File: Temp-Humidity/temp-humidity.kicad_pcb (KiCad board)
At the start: 2 copper layers, 34 x 74 mm, 30 parts, among them IC1 ATMEGA328P-A, P1 BATTERY, P2 CONN_02X03, P3 SERIAL/DEBUG, P4 ANTENNA, SW1 SW_PUSH_SMALL_H, U1 AT25DF512, U2 HDC1080, U3 ATSHA204A, U4 NRF24L01, U5 RFM69HW, Y1 12MHz

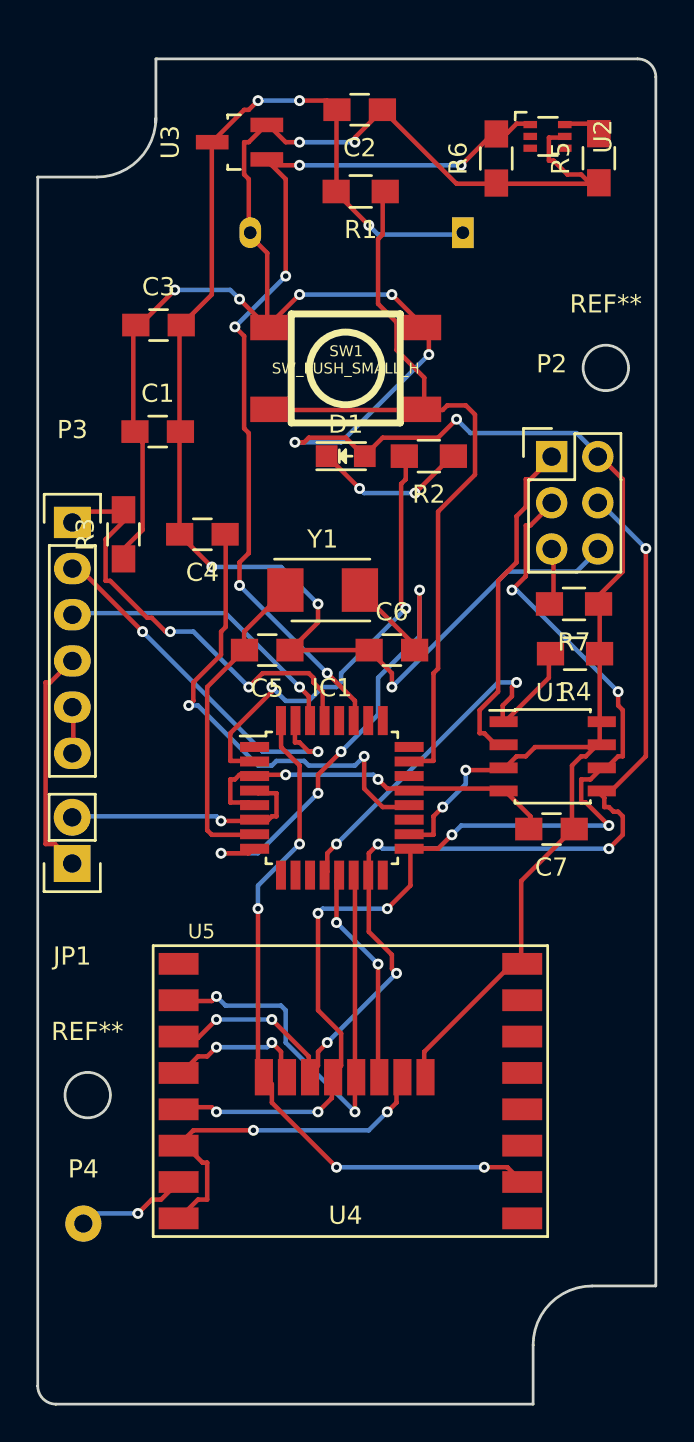
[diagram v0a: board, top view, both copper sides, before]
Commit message: More work on hum/temp
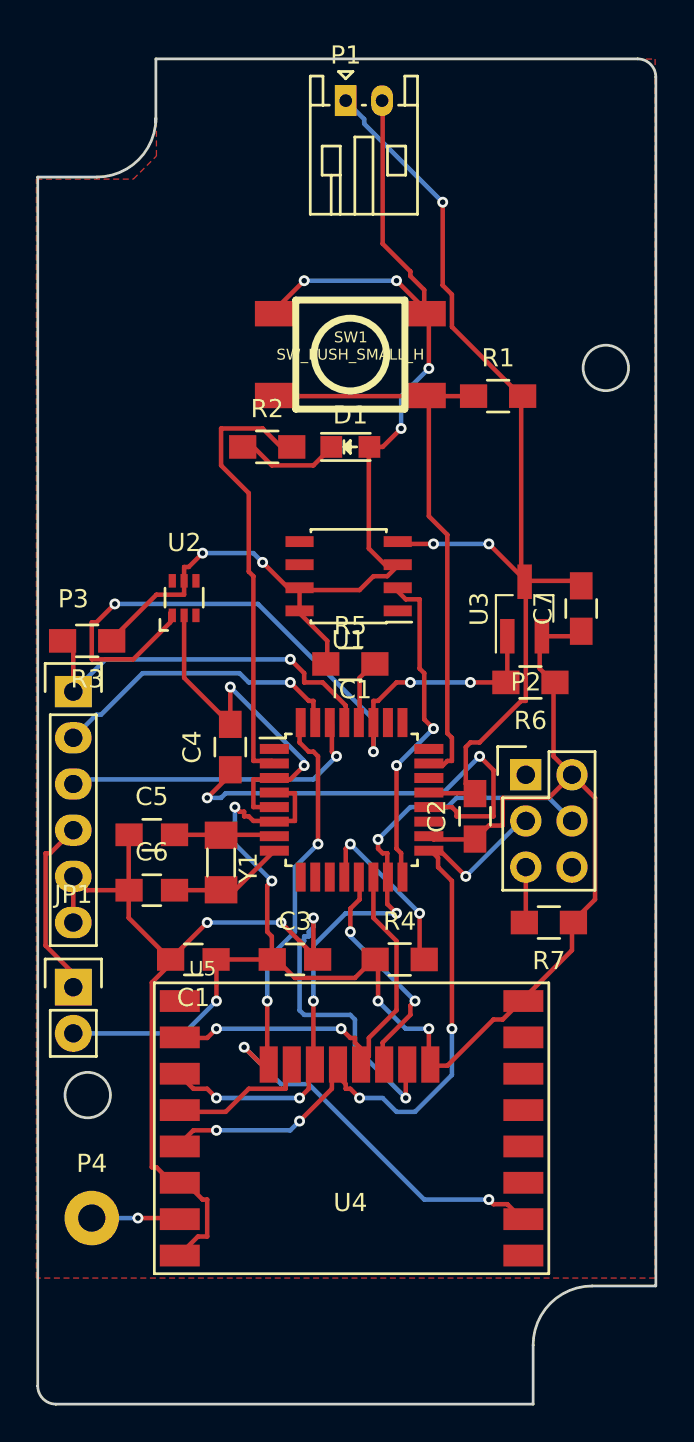
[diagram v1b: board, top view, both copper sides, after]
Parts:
- removed REF** (x2): MountingHole_2.5mm, Mounting_Holes:MountingHole_2.5mm
- P1: moved to F.Cu
- Y1: footprint Crystals:Crystal_SMD_5032_2Pads -> mysensors_obscurities:XTAL_3.2x1.5mm
- moved C2 39.4 mm to (135.1, 87.4), turned to 90 degrees
- moved C3 35.7 mm to (125.2, 95.2)
- moved U2 32.3 mm to (119.1, 75.4), turned to 0 degrees
- moved R5 31.0 mm to (128.3, 79.0), turned to 0 degrees
- moved U3 30.1 mm to (137.9, 76.0)
- moved C1 29.1 mm to (119.6, 95.2), turned to 180 degrees
- moved R6 28.9 mm to (138.2, 80.0), turned to 180 degrees
- moved R4 19.4 mm to (131.0, 95.2), turned to 0 degrees
- moved C6 18.7 mm to (117.3, 91.4)
- moved R7 17.6 mm to (139.2, 93.2)
- moved P2 17.6 mm to (137.9, 85.1)
- moved Y1 16.0 mm to (121.2, 89.9), turned to 270 degrees
- moved U1 15.0 mm to (128.2, 74.2), turned to 180 degrees
- moved R1 13.6 mm to (136.4, 64.3), turned to 0 degrees
- moved P1 13.2 mm to (128.0, 48.0), turned to 0 degrees
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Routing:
- net Net-(C6-Pad2): track 30.2 -> 6.77 mm, vias 4 -> 0
- net /SCK: track 63.8 -> 40.5 mm, vias 8 -> 5
- net /MOSI: track 61.3 -> 38.3 mm, vias 7 -> 5
- net +3V3: track 173.3 -> 153.4 mm, vias 12 -> 11
- net GND: track 123.1 -> 142.0 mm, vias 10 -> 9
- net /FLASH_CS: track 23.6 -> 10.0 mm
- net /BTN1: track 46.9 -> 33.7 mm
- net Net-(C5-Pad2): track 17.8 -> 5.80 mm
- net /SDA: track 51.5 -> 41.5 mm, vias 6 -> 4
- net /TX: track 20.6 -> 16.7 mm, vias 2 -> 1
- net /DTR: track 24.4 -> 21.3 mm, vias 2 -> 1
- net /IRQ: track 38.7 -> 41.8 mm
- net /CSN: track 26.8 -> 23.8 mm
- net VDD: track 13.1 -> 10.0 mm
- net Net-(D1-Pad1): track 8.65 -> 5.78 mm, vias 2 -> 0
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- removed copper zone on B.Cu, net GND
